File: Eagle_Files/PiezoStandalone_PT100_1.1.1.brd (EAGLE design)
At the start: 42.9 x 15.4 mm, 69 parts, among them J1 CON-MOLEX-4P-1.25MM048, U1 ATMEGA48PA-MMHR28M1-L, U2 L78L05ACU, U3 LM2902QT

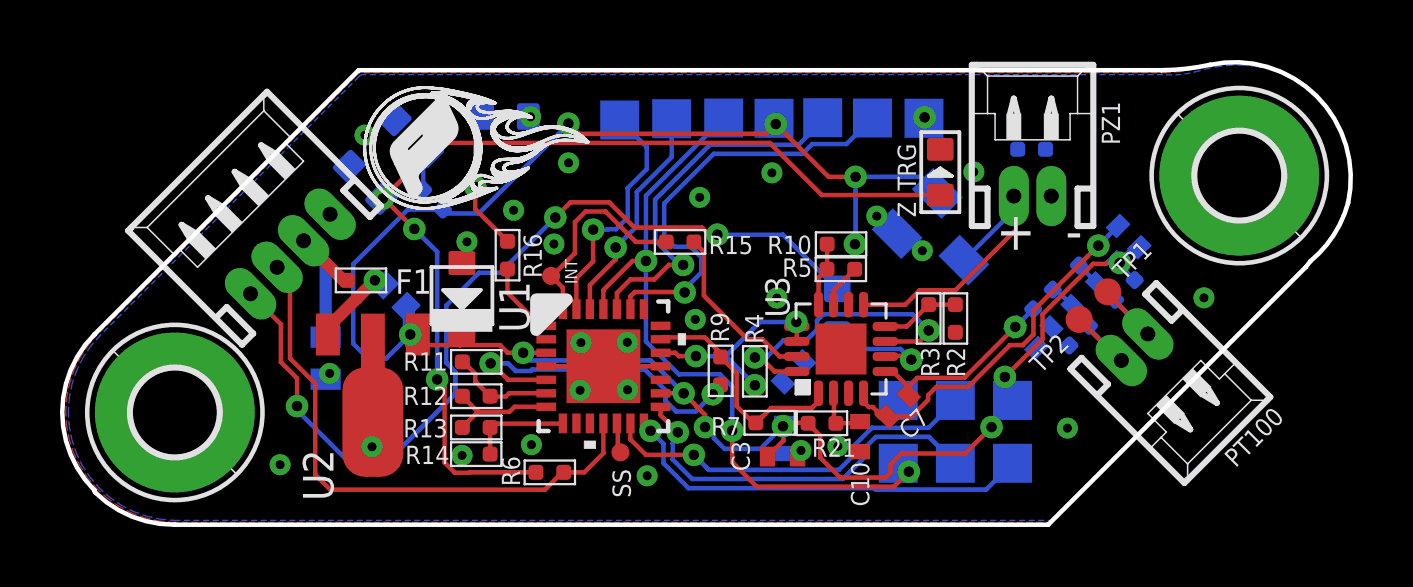
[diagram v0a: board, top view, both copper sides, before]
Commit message: Fixed airwires and overlaps
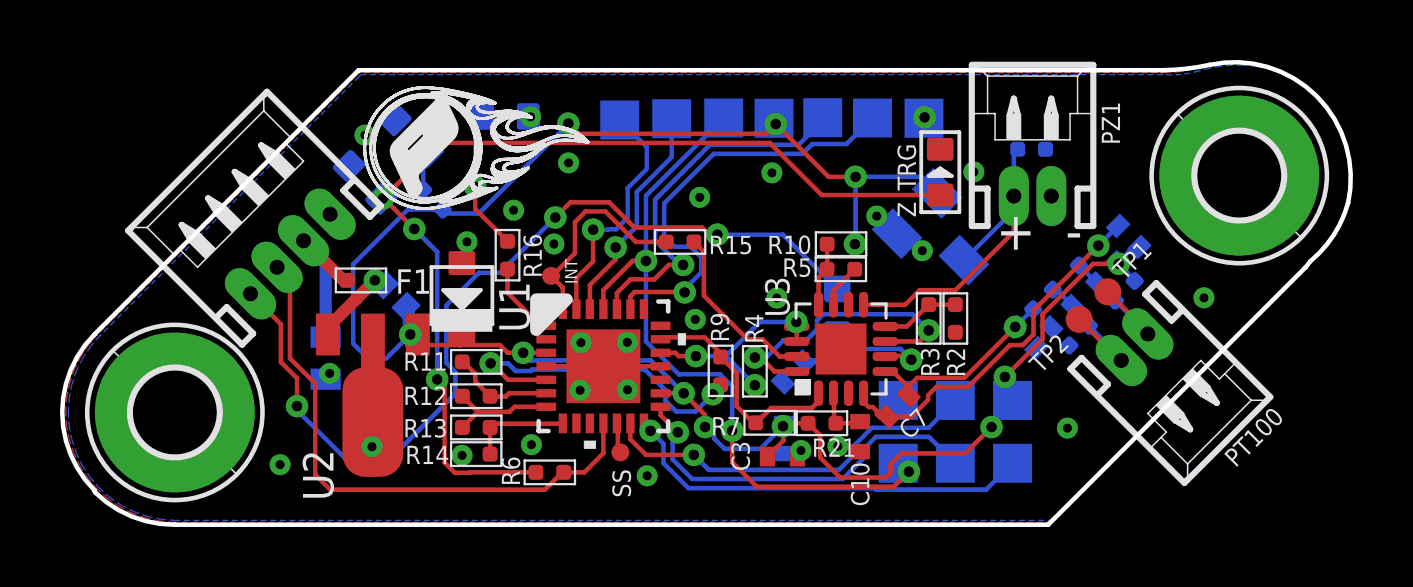
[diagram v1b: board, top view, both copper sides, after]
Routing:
- net PZ+: track 8.66 -> 11.8 mm
- net PT_IN-: track 5.35 -> 6.87 mm
- net PT100_JUMP: track 1.02 -> 1.74 mm

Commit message: Fixed spacing for zener diode
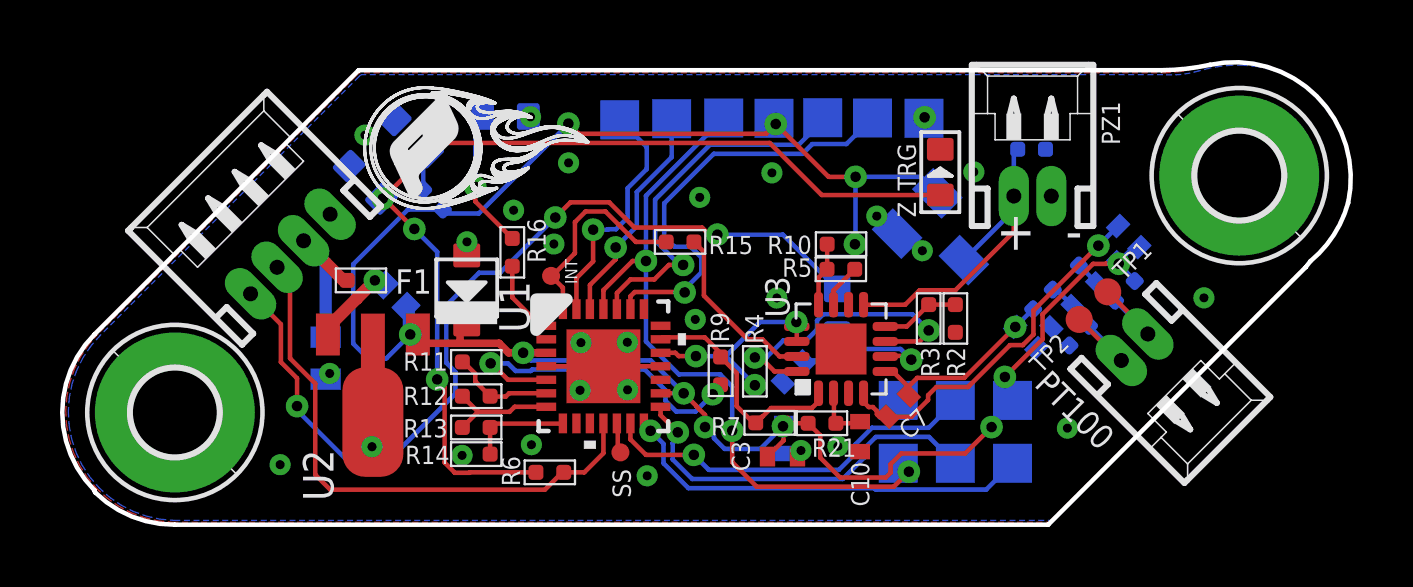
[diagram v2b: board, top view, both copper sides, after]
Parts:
- moved D1 0.30 mm to (14.2, 7.68)
- moved R16 0.19 mm to (15.7, 8.94)
